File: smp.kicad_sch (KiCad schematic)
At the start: 13 parts

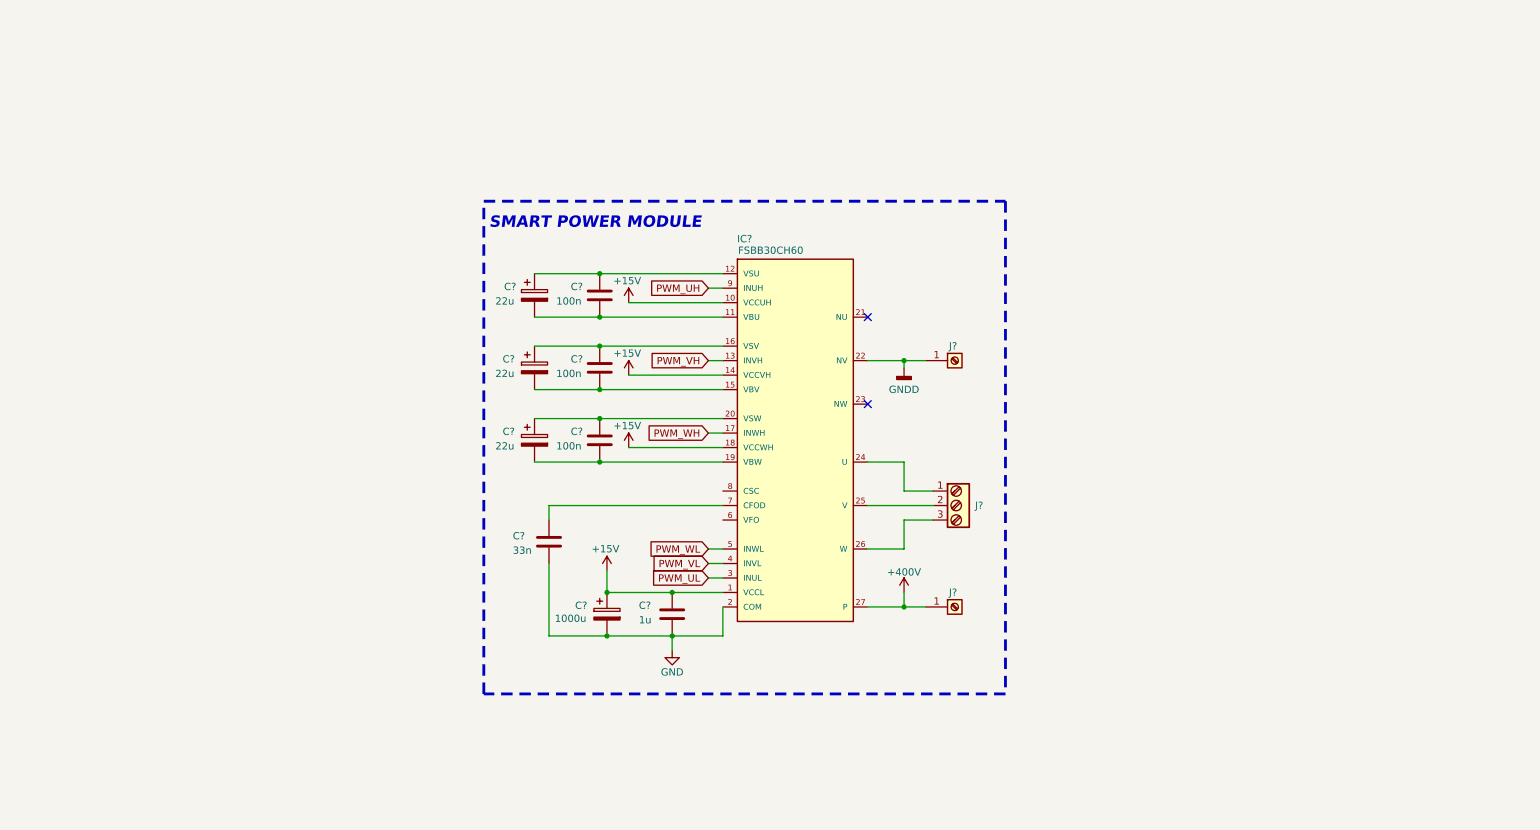
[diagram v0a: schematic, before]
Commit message: midsave
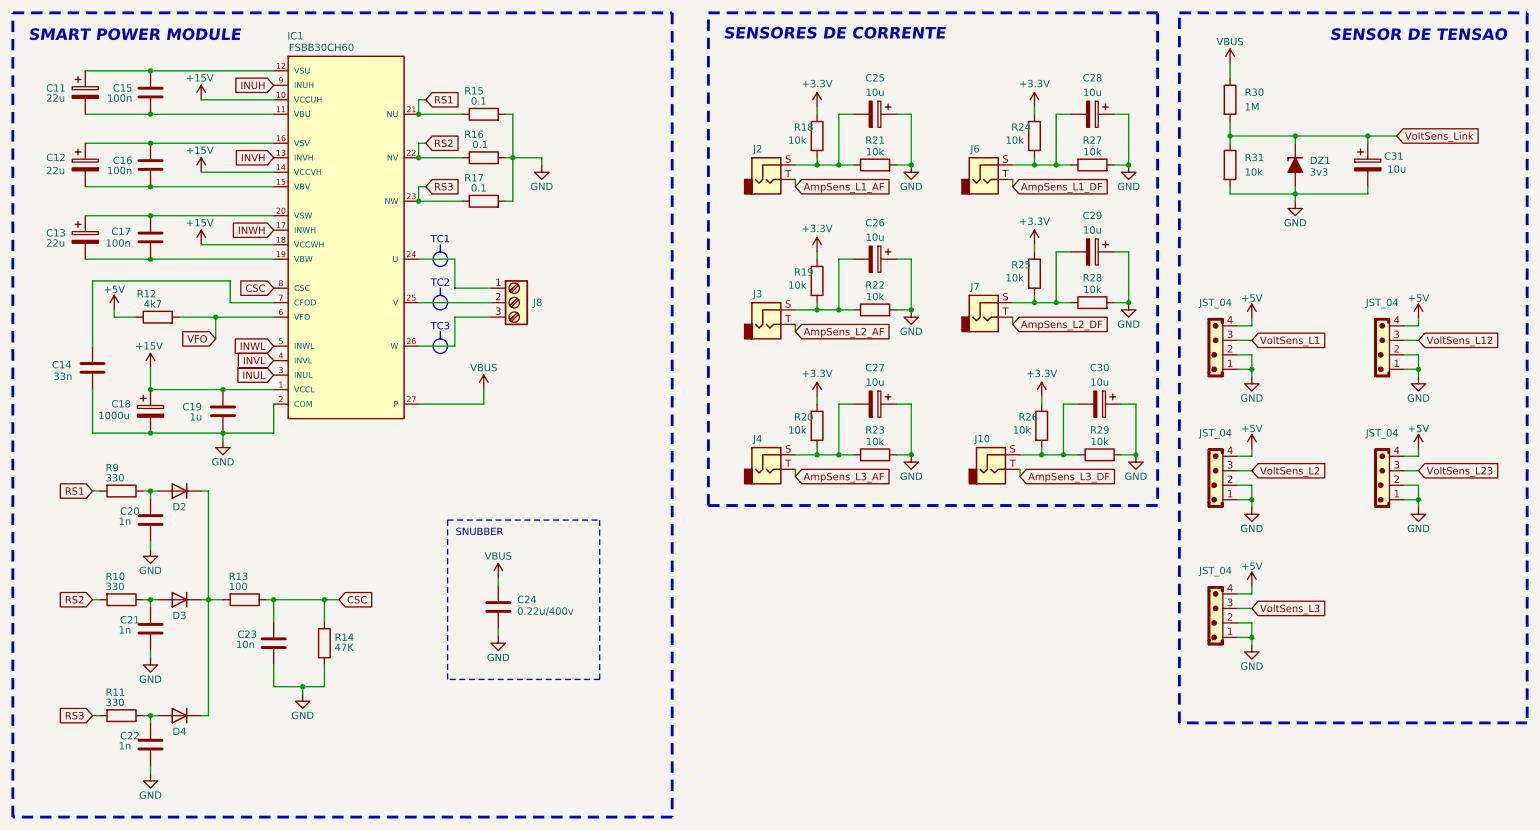
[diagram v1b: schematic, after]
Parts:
- removed J? (x2): Screw_Terminal_01x01, symbol Connector:Screw_Terminal_01x01
- added C20, C21, C22: 1n, Capacitor_THT:C_Disc_D4.7mm_W2.5mm_P5.00mm, symbol Device:C
- added C23: 10n, Capacitor_THT:C_Disc_D4.7mm_W2.5mm_P5.00mm, symbol Device:C
- added C24: 0.22u/400v, Capacitor_THT:C_Rect_L13.5mm_W5.0mm_P10.00mm_FKS3_FKP3_MKS4, symbol Device:C
- added C25, C26, C27, C28, C29, C30, C31: 10u, Capacitor_THT:CP_Radial_D6.3mm_P2.50mm, symbol Device:C_Polarized
- added D2, D3, D4: ~, Diode_THT:D_DO-15_P15.24mm_Horizontal, symbol Device:D
- added DZ1: 3v3, Diode_THT:D_DO-15_P15.24mm_Horizontal, symbol PCM_Diode_Zener_AKL:D_Zener_Generic
- added J10, J2, J3, J4, J6, J7: AudioJack2, Connector_Audio:Jack_3.5mm_CUI_SJ1-3525N_Horizontal, symbol Connector_Audio:AudioJack2
- added J11, J12, J13, J14, J15: JST_04, Connector_JST:JST_EH_B4B-EH-A_1x04_P2.50mm_Vertical, symbol PCM_SL_Connectors:JST_04
- added R10, R11, R9: 330, PCM_Resistor_THT_AKL:R_Axial_DIN0411_L9.9mm_D3.6mm_P20.32mm_Horizontal, symbol Device:R
- added R12: 4k7, PCM_Resistor_THT_AKL:R_Axial_DIN0411_L9.9mm_D3.6mm_P20.32mm_Horizontal, symbol Device:R
- added R13: 100, PCM_Resistor_THT_AKL:R_Axial_DIN0411_L9.9mm_D3.6mm_P20.32mm_Horizontal, symbol Device:R
- added R14: 47K, PCM_Resistor_THT_AKL:R_Axial_DIN0411_L9.9mm_D3.6mm_P20.32mm_Horizontal, symbol Device:R
- added R15, R16, R17: 0.1, PCM_Resistor_THT_AKL:R_Axial_DIN0922_L20.0mm_D9.0mm_P30.48mm_Horizontal, symbol Device:R
- added R18, R19, R20, R21, R22, R23, R24, R25, R26, R27, R28, R29, R31: 10k, PCM_Resistor_THT_AKL:R_Axial_DIN0411_L9.9mm_D3.6mm_P20.32mm_Horizontal, symbol Device:R
- added R30: 1M, PCM_Resistor_THT_AKL:R_Axial_DIN0411_L9.9mm_D3.6mm_P20.32mm_Horizontal, symbol Device:R
- C11, C12, C13: renamed from C?; footprint (none) -> Capacitor_THT:CP_Radial_D6.3mm_P2.50mm
- C14: renamed from C?; footprint (none) -> Capacitor_THT:C_Disc_D6.0mm_W2.5mm_P5.00mm
- C15, C16, C17, C19: renamed from C?; footprint (none) -> Capacitor_THT:C_Disc_D4.7mm_W2.5mm_P5.00mm
- C18: renamed from C?; footprint (none) -> Capacitor_THT:CP_Radial_D14.0mm_P5.00mm
- gave numbers to parts that had none: 2
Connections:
- net GND: now also C20.2, C21.2, C22.2, C23.2, C24.2, C25.1, C26.1, C27.1, C28.1, C29.1, C30.1, C31.2, DZ1.2 (A), J11.1, J11.2, J12.1, J12.2, J13.1, J13.2, J14.1, J14.2, J15.1, J15.2, R14.2, R15.2, R16.2, R17.2, R21.2, R22.2, R23.2, R27.2, R28.2, R29.2, R31.2
- net RS1: now reaches IC1.21 (NU)
- net RS1: now also R15.1, R9.2
- net RS3: now reaches IC1.23 (NW)
- net RS3: now also R11.2, R17.1
- net VFO: now reaches IC1.6 (VFO)
- net VFO: now also R12.2
- net CSC: now reaches IC1.8 (CSC)
- net CSC: now also C23.1, R13.1, R14.1
- net +400V renamed VBUS
- net VBUS: now also C24.1, R30.1
- net GNDD renamed RS2
- net RS2: now also R10.2, R16.1
- net PWM_UH renamed INUH
- net PWM_UL renamed INUL
- net PWM_VH renamed INVH
- net PWM_VL renamed INVL
- net PWM_WH renamed INWH
- net PWM_WL renamed INWL
- new net: C20.1, D2.2 (A), R9.1
- new net: C28.2, J6.S, R24.2, R27.1
- new net: D2.1 (K), D3.1 (K), D4.1 (K), R13.2
- new net: C21.1, D3.2 (A), R10.1
- new net: C27.2, J4.S, R20.2, R23.1
- new net: C30.2, J10.S, R26.2, R29.1
- new net: C26.2, J3.S, R19.2, R22.1
- new net: C25.2, J2.S, R18.2, R21.1
- new net: C29.2, J7.S, R25.2, R28.1
- new net: C22.1, D4.2 (A), R11.1
- new net +3.3V: R18.1, R19.1, R20.1, R24.1, R25.1, R26.1
- new net +5V: J11.4, J12.4, J13.4, J14.4, J15.4, R12.1
- new net AmpSens_L1_AF: J2.T
- new net AmpSens_L1_DF: J6.T
- new net AmpSens_L2_AF: J3.T
- new net AmpSens_L2_DF: J7.T
- new net AmpSens_L3_AF: J4.T
- new net AmpSens_L3_DF: J10.T
- new net VoltSens_L1: J11.3
- new net VoltSens_L12: J14.3
- new net VoltSens_L2: J12.3
- new net VoltSens_L23: J15.3
- new net VoltSens_L3: J13.3
- new net VoltSens_Link: C31.1, DZ1.1 (K), R30.2, R31.1
- no-connect marks 2 -> 0
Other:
- note added: "SENSOR DE TENSAO"
- note added: "SENSORES DE CORRENTE"
- note added: "SNUBBER"
- note added: "TC1"
- note added: "TC2"
- note added: "TC3"
- company: (none) -> Autor: José Fonseca
- title: (none) -> Smart Power Module
- moved on the sheet: C11, C12, C13, C14, C15, C16, C17, C18, C19, IC1, J8
